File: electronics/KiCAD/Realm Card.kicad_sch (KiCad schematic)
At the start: 22 parts, among them J1 Conn_02x07_Top_Bottom, J2 Micro_SD_Card, J3 Conn_01x02_Female, J4 Conn_02x25_Top_Bottom, SW1 SW_SPDT, U1 MCP73831-2-OT, U2 MCP100-315D

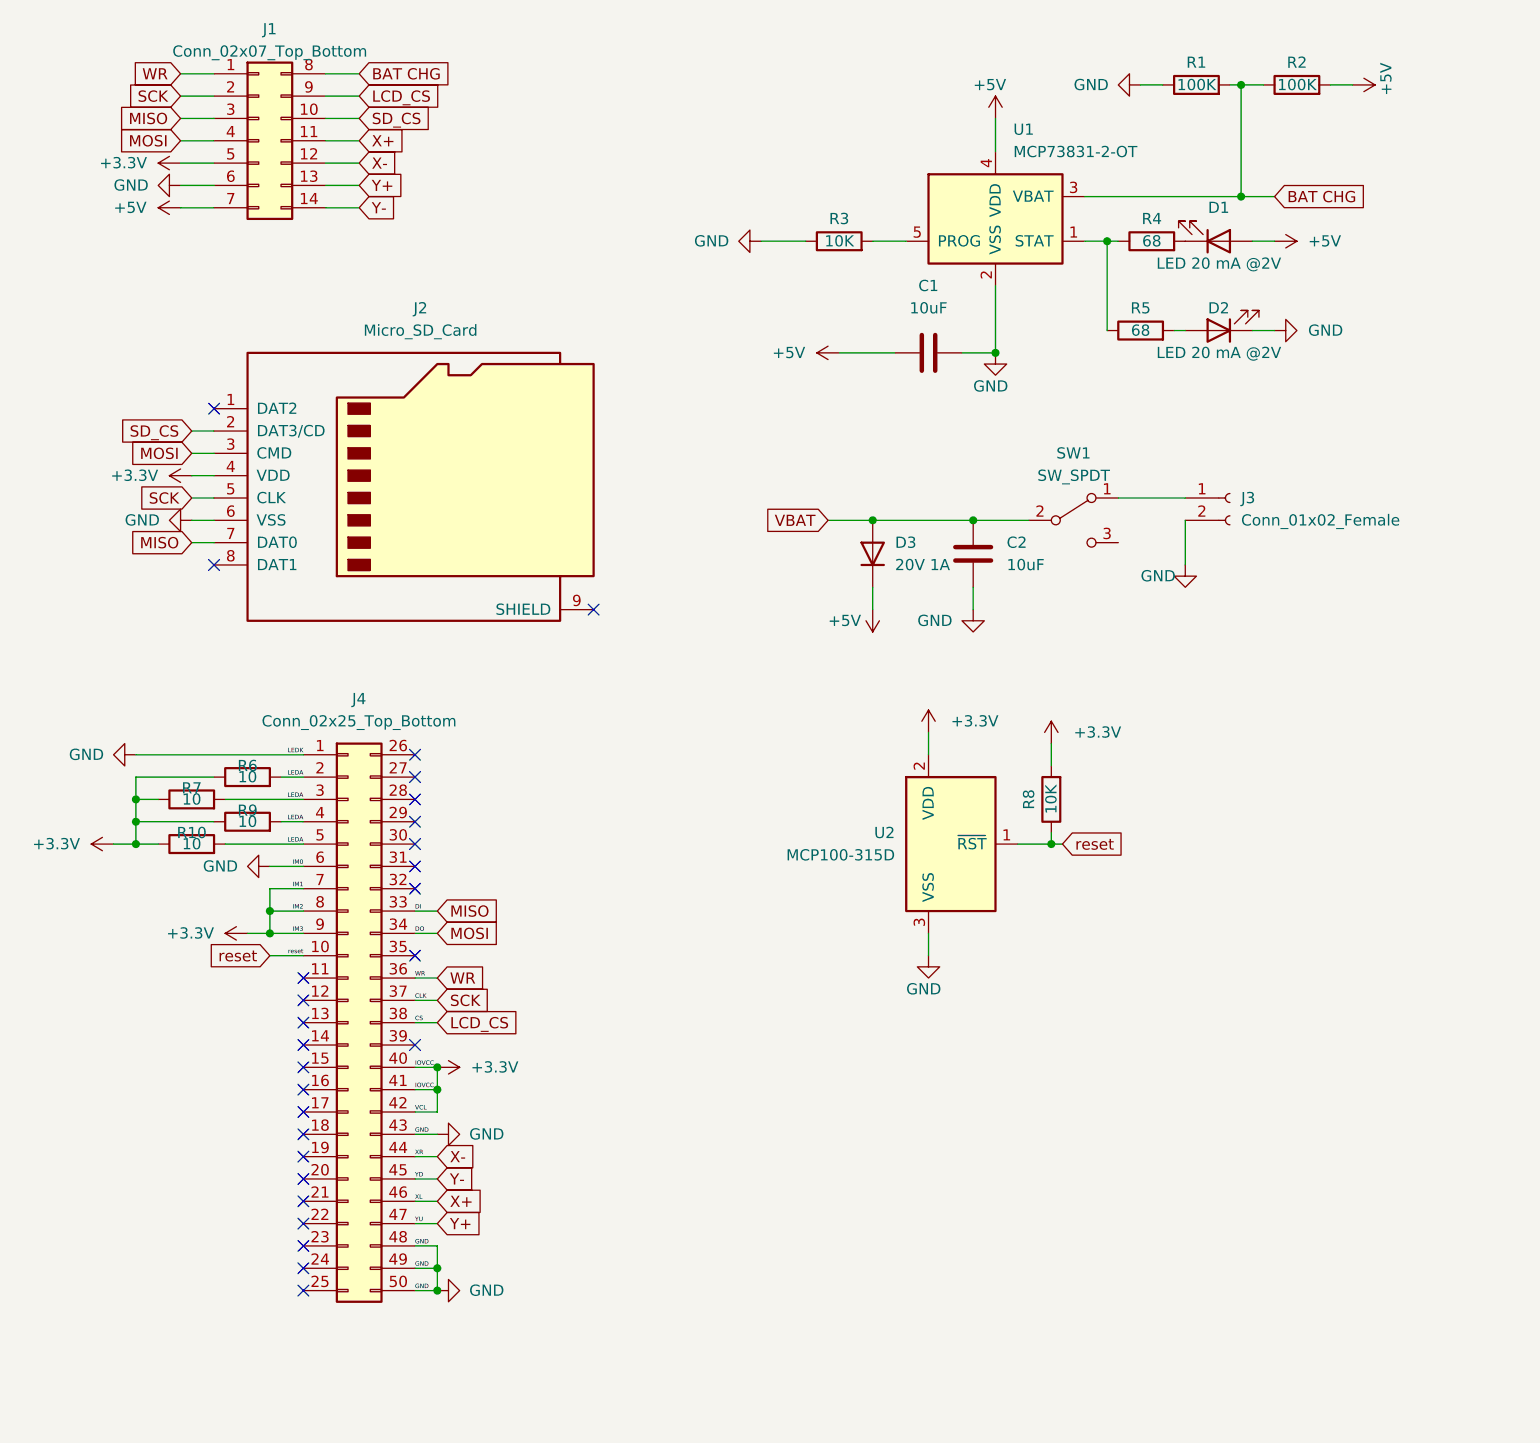
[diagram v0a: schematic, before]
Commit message: updated board
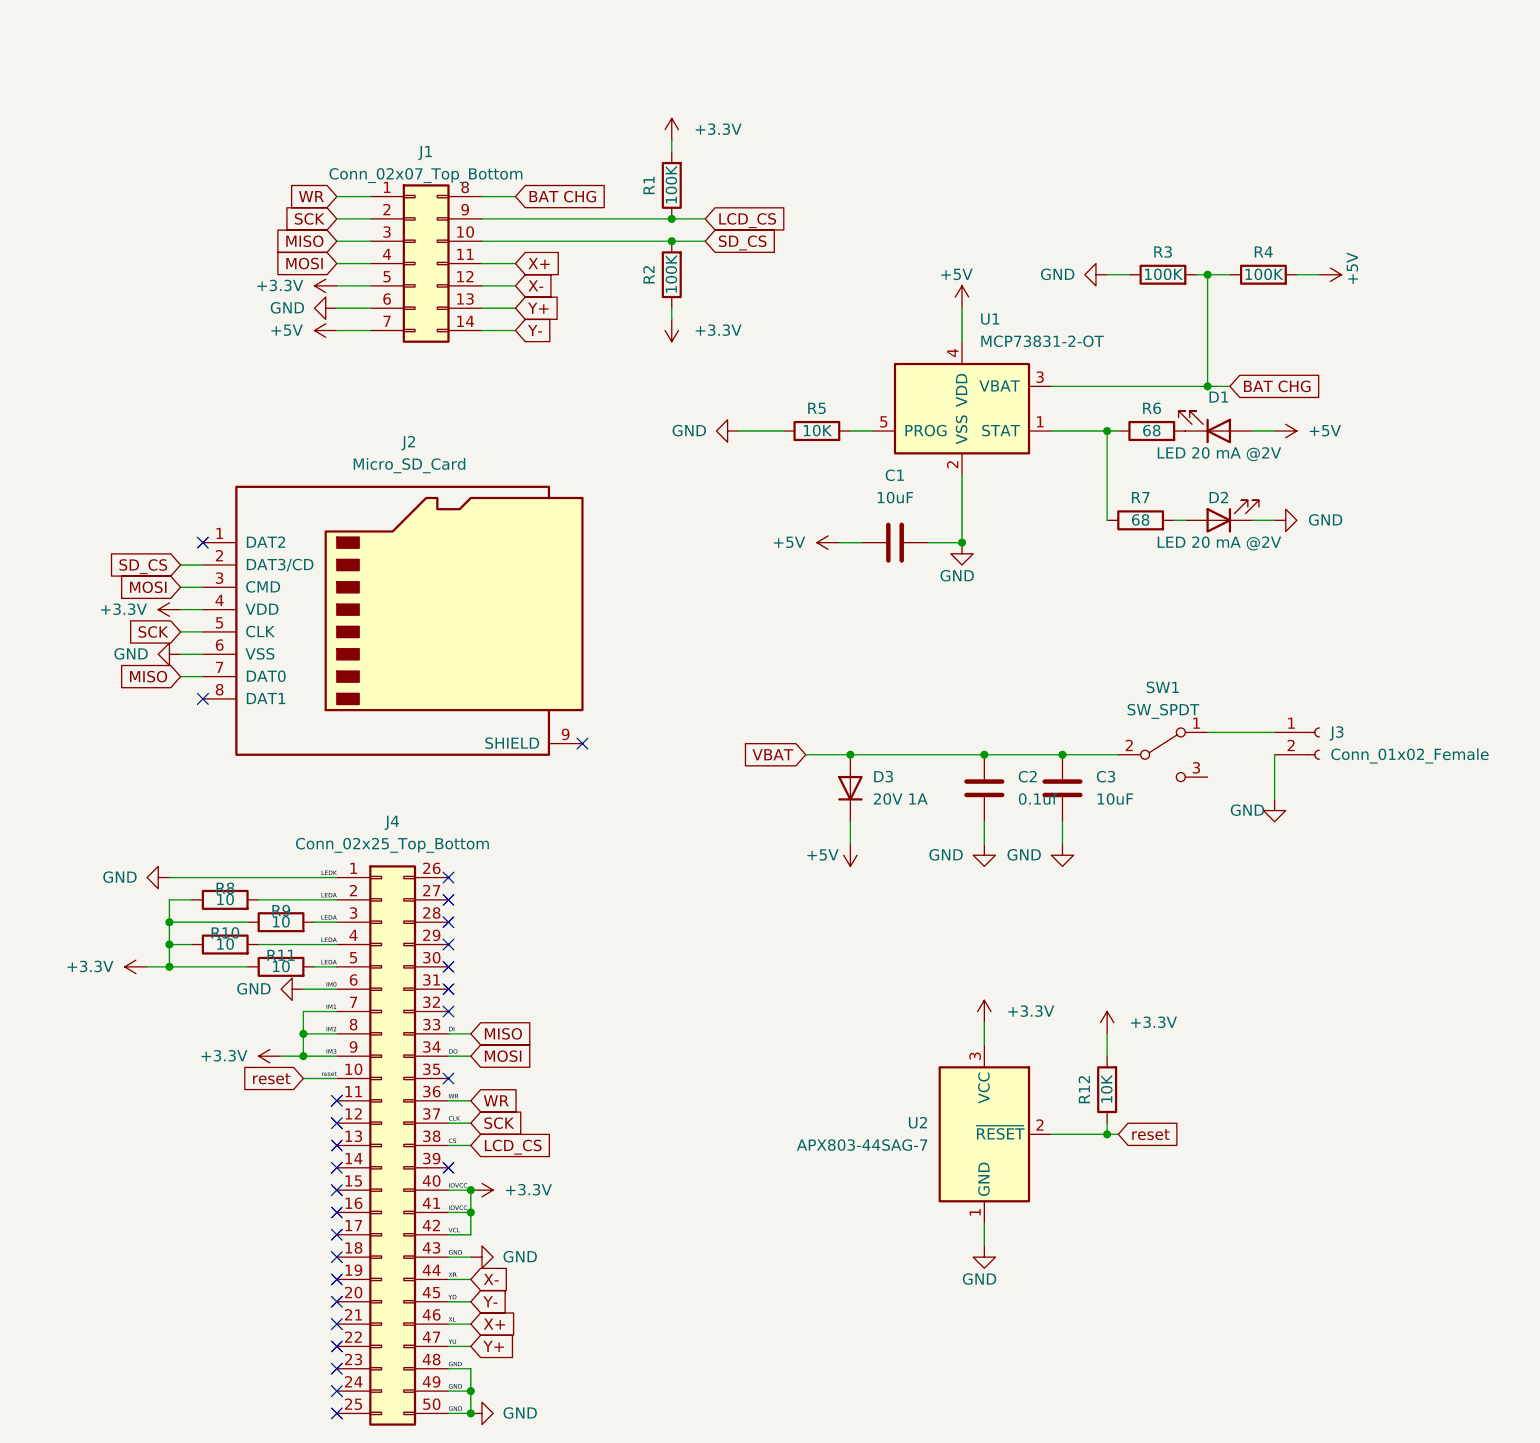
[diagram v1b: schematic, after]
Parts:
- removed U2: MCP100-315D, Package_TO_SOT_SMD:SOT-23, symbol Power_Supervisor:MCP100-315D
- added C2: 0.1uf, Capacitor_SMD:C_0805_2012Metric, symbol Device:C
- added R1, R2: 100K, Resistor_SMD:R_0805_2012Metric, symbol Device:R
- added U2: APX803-44SAG-7, Package_TO_SOT_SMD:SOT-23, symbol Power_Supervisor:LM809
- renumbered C2 to C3, R7 to R10, R6 to R11, R8 to R12, R1 to R3, R2 to R4, R3 to R5, R4 to R6, R5 to R7, R10 to R8
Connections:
- net +3.3V: now also R1.2, R2.1, U2.3 (VCC)
- net GND: now also C2.1, U2.1 (GND)
- net LCD_CS: now also R1.1
- net SD_CS: now also R2.2
- net VBAT: now also C2.2
- net reset: now also U2.2 (~{RESET})
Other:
- moved on the sheet: C1, C3, D1, D2, D3, J1, J2, J3, J4, R10, R11, R12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

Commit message: revised code
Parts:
- U2: LCSC C155243 -> C9965
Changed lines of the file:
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@@
       (effects (font (size 1.27 1.27)) hide)
     )
-    (property "LCSC" "C155243" (id 5) (at 118.11 134.62 0)
+    (property "LCSC" "C9965" (id 5) (at 118.11 134.62 0)
       (effects (font (size 1.27 1.27)) hide)
     )
